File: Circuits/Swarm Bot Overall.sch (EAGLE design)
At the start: 7 parts, among them IC1 MEGA164P/324P/644P-AU, IC2 MCP73831

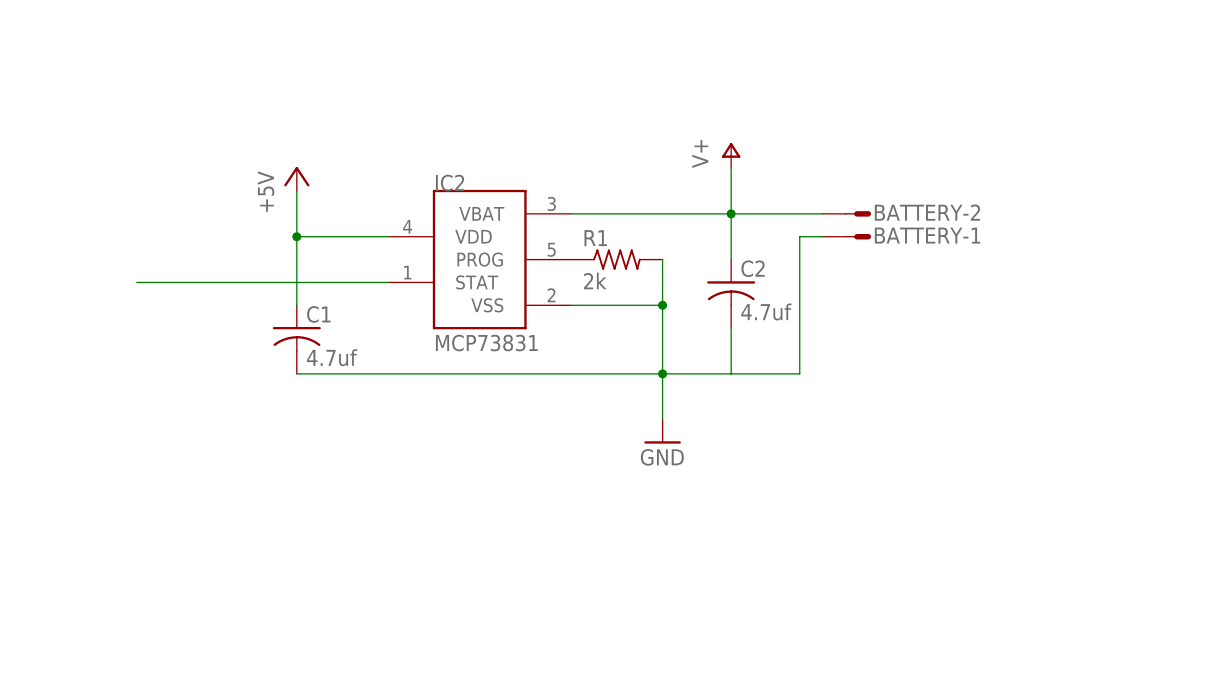
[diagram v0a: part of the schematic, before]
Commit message: Finished Charger?
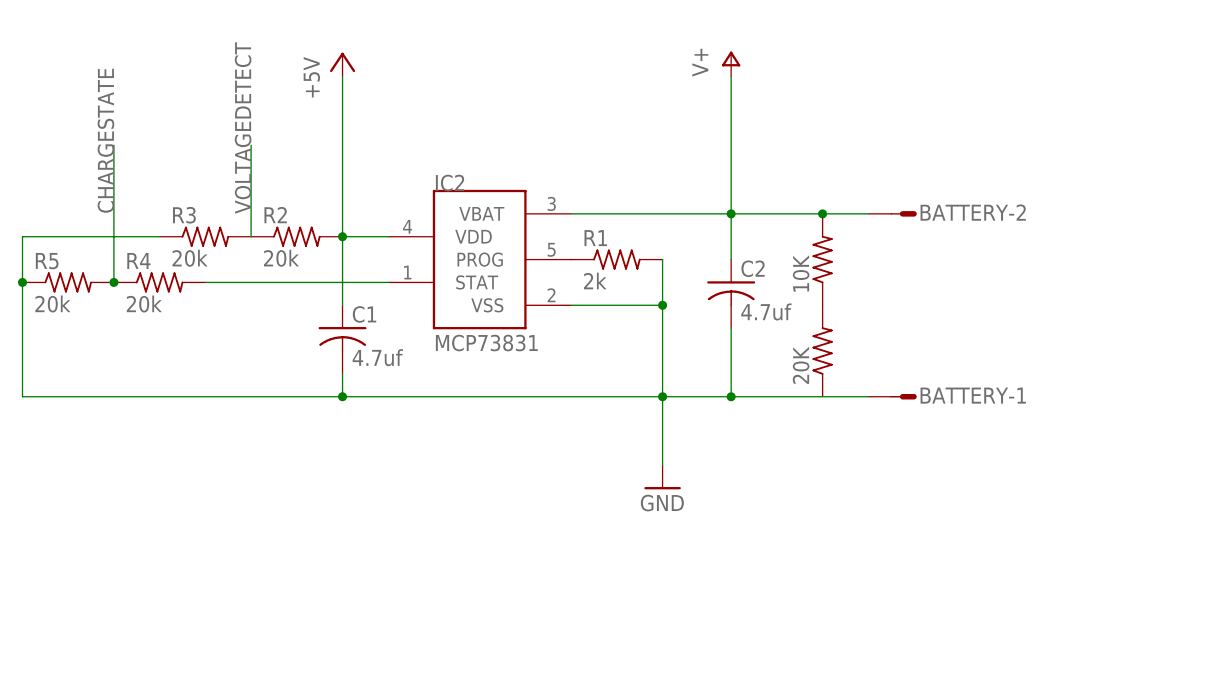
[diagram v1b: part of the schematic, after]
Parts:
- added 10K, 20K: (no value), resistor:R-US_0204/5
- added R2, R3, R4, R5: 20k, resistor:R-US_0204/5
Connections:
- new net CHARGESTATE: R4.1, R5.2
- new net N$6: IC2.STAT, R4.2
- new net VOLTAGEDETECT: R2.1, R3.2
- net +5V: now also R2.2
- net GND: now also R3.1, R5.1
- net N$3: now also 10K.1, 20K.2; no longer IC2.STAT
- net V+: now also 10K.2
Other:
- moved on the sheet: BATTERY-1, BATTERY-2, C1
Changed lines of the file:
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@@
 <part name="FTDI" library="con-amp-quick" deviceset="M03S" device=""/>
 <part name="GND3" library="supply1" deviceset="GND" device=""/>
+<part name="R2" library="resistor" deviceset="R-US_" device="0204/5" value="20k"/>
+<part name="R3" library="resistor" deviceset="R-US_" device="0204/5" value="20k"/>
+<part name="R4" library="resistor" deviceset="R-US_" device="0204/5" value="20k"/>
+<part name="R5" library="resistor" deviceset="R-US_" device="0204/5" value="20k"/>
+<part name="10K" library="resistor" deviceset="R-US_" device="0204/5"/>
+<part name="20K" library="resistor" deviceset="R-US_" device="0204/5"/>
 </parts>
 <sheets>
@@
 <instance part="IC2" gate="G$1" x="-104.14" y="165.1"/>
 <instance part="R1" gate="G$1" x="-88.9" y="165.1"/>
-<instance part="C1" gate="G$1" x="-124.46" y="157.48"/>
-<instance part="GND2" gate="1" x="-83.82" y="144.78"/>
-<instance part="P+1" gate="1" x="-124.46" y="175.26"/>
+<instance part="C1" gate="G$1" x="-119.38" y="157.48"/>
+<instance part="GND2" gate="1" x="-83.82" y="139.7"/>
+<instance part="P+1" gate="1" x="-119.38" y="187.96"/>
 <instance part="C2" gate="G$1" x="-76.2" y="162.56"/>
-<instance part="P+2" gate="1" x="-76.2" y="177.8"/>
-<instance part="BATTERY" gate="-1" x="-60.96" y="167.64" rot="R180"/>
-<instance part="BATTERY" gate="-2" x="-60.96" y="170.18" rot="R180"/>
+<instance part="P+2" gate="1" x="-76.2" y="187.96"/>
+<instance part="BATTERY" gate="-1" x="-55.88" y="149.86" rot="R180"/>
+<instance part="BATTERY" gate="-2" x="-55.88" y="170.18" rot="R180"/>
 <instance part="FTDI" gate="-1" x="226.06" y="73.66" rot="R180"/>
 <instance part="FTDI" gate="-2" x="226.06" y="76.2" rot="R180"/>
 <instance part="FTDI" gate="-3" x="226.06" y="78.74" rot="R180"/>
 <instance part="GND3" gate="1" x="218.44" y="68.58"/>
+<instance part="R2" gate="G$1" x="-124.46" y="167.64"/>
+<instance part="R3" gate="G$1" x="-134.62" y="167.64"/>
+<instance part="R4" gate="G$1" x="-139.7" y="162.56"/>
+<instance part="R5" gate="G$1" x="-149.86" y="162.56"/>
+<instance part="10K" gate="G$1" x="-66.04" y="165.1" rot="R90"/>
+<instance part="20K" gate="G$1" x="-66.04" y="154.94" rot="R90"/>
 </instances>
 <busses>
@@
 <wire x1="-93.98" y1="160.02" x2="-83.82" y2="160.02" width="0.1524" layer="91"/>
 <wire x1="-83.82" y1="165.1" x2="-83.82" y2="160.02" width="0.1524" layer="91"/>
-<wire x1="-83.82" y1="160.02" x2="-83.82" y2="152.4" width="0.1524" layer="91"/>
-<wire x1="-83.82" y1="152.4" x2="-124.46" y2="152.4" width="0.1524" layer="91"/>
+<wire x1="-83.82" y1="160.02" x2="-83.82" y2="149.86" width="0.1524" layer="91"/>
+<wire x1="-83.82" y1="149.86" x2="-83.82" y2="142.24" width="0.1524" layer="91"/>
+<junction x="-83.82" y="160.02"/>
+<junction x="-83.82" y="149.86"/>
+<pinref part="GND2" gate="1" pin="GND"/>
+<wire x1="-83.82" y1="149.86" x2="-76.2" y2="149.86" width="0.1524" layer="91"/>
+<pinref part="C2" gate="G$1" pin="2"/>
+<wire x1="-76.2" y1="149.86" x2="-76.2" y2="157.48" width="0.1524" layer="91"/>
 <pinref part="C1" gate="G$1" pin="2"/>
-<wire x1="-83.82" y1="152.4" x2="-83.82" y2="147.32" width="0.1524" layer="91"/>
-<junction x="-83.82" y="160.02"/>
-<junction x="-83.82" y="152.4"/>
-<pinref part="GND2" gate="1" pin="GND"/>
-<wire x1="-83.82" y1="152.4" x2="-76.2" y2="152.4" width="0.1524" layer="91"/>
-<pinref part="C2" gate="G$1" pin="2"/>
-<wire x1="-76.2" y1="152.4" x2="-76.2" y2="157.48" width="0.1524" layer="91"/>
-<wire x1="-76.2" y1="152.4" x2="-68.58" y2="152.4" width="0.1524" layer="91"/>
-<wire x1="-68.58" y1="167.64" x2="-68.58" y2="152.4" width="0.1524" layer="91"/>
+<wire x1="-119.38" y1="152.4" x2="-119.38" y2="149.86" width="0.1524" layer="91"/>
+<wire x1="-119.38" y1="149.86" x2="-83.82" y2="149.86" width="0.1524" layer="91"/>
+<pinref part="R3" gate="G$1" pin="1"/>
+<wire x1="-139.7" y1="167.64" x2="-154.94" y2="167.64" width="0.1524" layer="91"/>
+<wire x1="-154.94" y1="167.64" x2="-154.94" y2="162.56" width="0.1524" layer="91"/>
+<wire x1="-154.94" y1="162.56" x2="-154.94" y2="149.86" width="0.1524" layer="91"/>
+<wire x1="-154.94" y1="149.86" x2="-119.38" y2="149.86" width="0.1524" layer="91"/>
+<junction x="-119.38" y="149.86"/>
+<pinref part="R5" gate="G$1" pin="1"/>
+<junction x="-154.94" y="162.56"/>
 <pinref part="BATTERY" gate="-1" pin="S"/>
-<wire x1="-66.04" y1="167.64" x2="-68.58" y2="167.64" width="0.1524" layer="91"/>
+<wire x1="-76.2" y1="149.86" x2="-60.96" y2="149.86" width="0.1524" layer="91"/>
+<junction x="-76.2" y="149.86"/>
 </segment>
 <segment>
@@
 </segment>
 </net>
-<net name="N$3" class="0">
-<segment>
-<pinref part="IC2" gate="G$1" pin="STAT"/>
-<wire x1="-114.3" y1="162.56" x2="-142.24" y2="162.56" width="0.1524" layer="91"/>
-</segment>
-</net>
 <net name="+5V" class="0">
 <segment>
 <pinref part="IC2" gate="G$1" pin="VDD"/>
 <pinref part="C1" gate="G$1" pin="1"/>
-<wire x1="-114.3" y1="167.64" x2="-124.46" y2="167.64" width="0.1524" layer="91"/>
-<wire x1="-124.46" y1="167.64" x2="-124.46" y2="160.02" width="0.1524" layer="91"/>
-<wire x1="-124.46" y1="167.64" x2="-124.46" y2="172.72" width="0.1524" layer="91"/>
-<junction x="-124.46" y="167.64"/>
+<wire x1="-114.3" y1="167.64" x2="-119.38" y2="167.64" width="0.1524" layer="91"/>
+<wire x1="-119.38" y1="167.64" x2="-119.38" y2="160.02" width="0.1524" layer="91"/>
+<wire x1="-119.38" y1="167.64" x2="-119.38" y2="185.42" width="0.1524" layer="91"/>
+<junction x="-119.38" y="167.64"/>
 <pinref part="P+1" gate="1" pin="+5V"/>
+<pinref part="R2" gate="G$1" pin="2"/>
 </segment>
 </net>
@@
 <wire x1="-76.2" y1="170.18" x2="-93.98" y2="170.18" width="0.1524" layer="91"/>
 <wire x1="-76.2" y1="170.18" x2="-66.04" y2="170.18" width="0.1524" layer="91"/>
-<wire x1="-76.2" y1="170.18" x2="-76.2" y2="175.26" width="0.1524" layer="91"/>
+<wire x1="-66.04" y1="170.18" x2="-60.96" y2="170.18" width="0.1524" layer="91"/>
+<wire x1="-76.2" y1="170.18" x2="-76.2" y2="185.42" width="0.1524" layer="91"/>
 <junction x="-76.2" y="170.18"/>
 <pinref part="P+2" gate="1" pin="V+"/>
 <pinref part="BATTERY" gate="-2" pin="S"/>
+<pinref part="10K" gate="G$1" pin="2"/>
+<junction x="-66.04" y="170.18"/>
 </segment>
 </net>
@@
 </segment>
 </net>
+<net name="VOLTAGEDETECT" class="0">
+<segment>
+<pinref part="R2" gate="G$1" pin="1"/>
+<pinref part="R3" gate="G$1" pin="2"/>
+<wire x1="-129.54" y1="167.64" x2="-129.54" y2="177.8" width="0.1524" layer="91"/>
+<label x="-129.54" y="170.18" size="1.778" layer="95" rot="R90"/>
+</segment>
+</net>
+<net name="CHARGESTATE" class="0">
+<segment>
+<pinref part="R4" gate="G$1" pin="1"/>
+<pinref part="R5" gate="G$1" pin="2"/>
+<wire x1="-144.78" y1="162.56" x2="-144.78" y2="177.8" width="0.1524" layer="91"/>
+<label x="-144.78" y="170.18" size="1.778" layer="95" rot="R90"/>
+<junction x="-144.78" y="162.56"/>
+</segment>
+</net>
+<net name="N$6" class="0">
+<segment>
+<pinref part="R4" gate="G$1" pin="2"/>
+<pinref part="IC2" gate="G$1" pin="STAT"/>
+<wire x1="-134.62" y1="162.56" x2="-114.3" y2="162.56" width="0.1524" layer="91"/>
+</segment>
+</net>
+<net name="N$3" class="0">
+<segment>
+<pinref part="10K" gate="G$1" pin="1"/>
+<pinref part="20K" gate="G$1" pin="2"/>
+</segment>
+</net>
